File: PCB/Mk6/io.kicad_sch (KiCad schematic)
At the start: 10 parts, among them J11 DISPLAY, J6 PortA: 5V PA0 PA1 PA2 PA3 PA4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, J7 PortB: 5V PB0 PB1 PB2 PB3 PB4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, J8 Input Port, J9 Output Port, U11 R6522, U12 74LS573, U13 74LS574

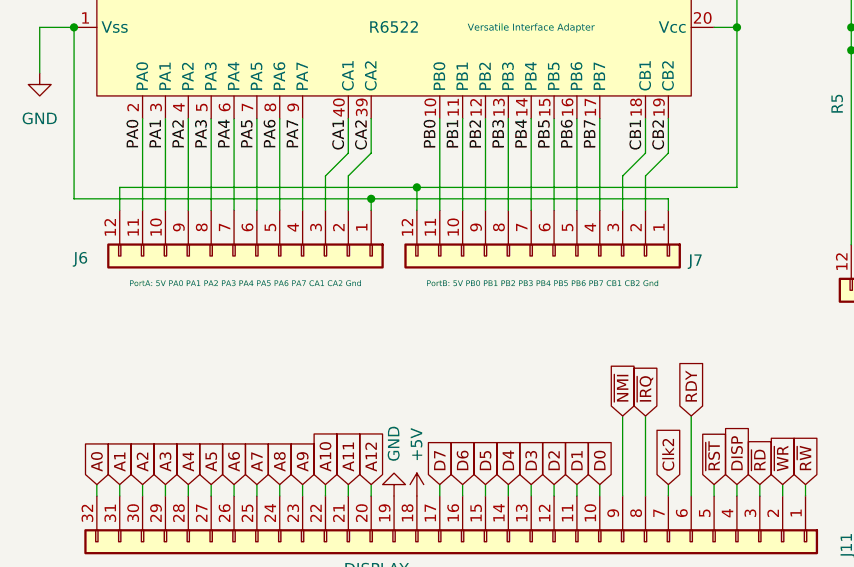
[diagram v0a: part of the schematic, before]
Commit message: cleanup
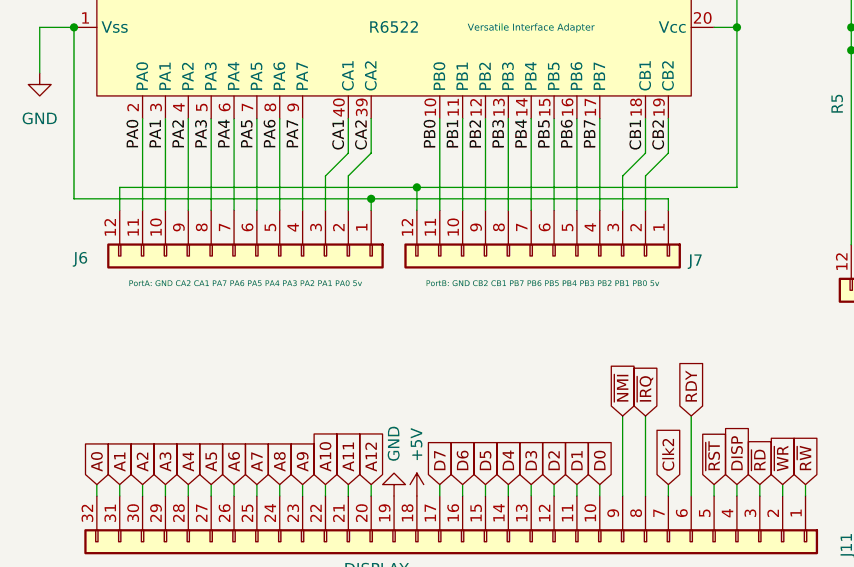
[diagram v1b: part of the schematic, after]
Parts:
- J6: value PortA: 5V PA0 PA1 PA2 PA3 PA4 PA5 PA6 PA7 CA1 CA2 Gnd -> PortA: GND CA2 CA1 PA7 PA6 PA5 PA4 PA3 PA2 PA1 PA0 5v
- J7: value PortB: 5V PB0 PB1 PB2 PB3 PB4 PB5 PB6 PB7 CB1 CB2 Gnd -> PortB: GND CB2 CB1 PB7 PB6 PB5 PB4 PB3 PB2 PB1 PB0 5v
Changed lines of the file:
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@@
 			)
 		)
-		(property "Value" "PortB: 5V PB0 PB1 PB2 PB3 PB4 PB5 PB6 PB7 CB1 CB2 Gnd"
+		(property "Value" "PortB: GND CB2 CB1 PB7 PB6 PB5 PB4 PB3 PB2 PB1 PB0 5v"
 			(at 74.93 86.868 90)
 			(effects
@@
 			)
 		)
-		(property "Value" "PortA: 5V PA0 PA1 PA2 PA3 PA4 PA5 PA6 PA7 CA1 CA2 Gnd"
+		(property "Value" "PortA: GND CA2 CA1 PA7 PA6 PA5 PA4 PA3 PA2 PA1 PA0 5v"
 			(at 41.91 86.868 90)
 			(effects
